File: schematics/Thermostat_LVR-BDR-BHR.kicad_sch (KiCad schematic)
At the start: 12 parts, among them J1 Dupont 6pin, J2 Dupont 6pin, SW1 Button Down, SW2 Button Up, SW3 Button Enter

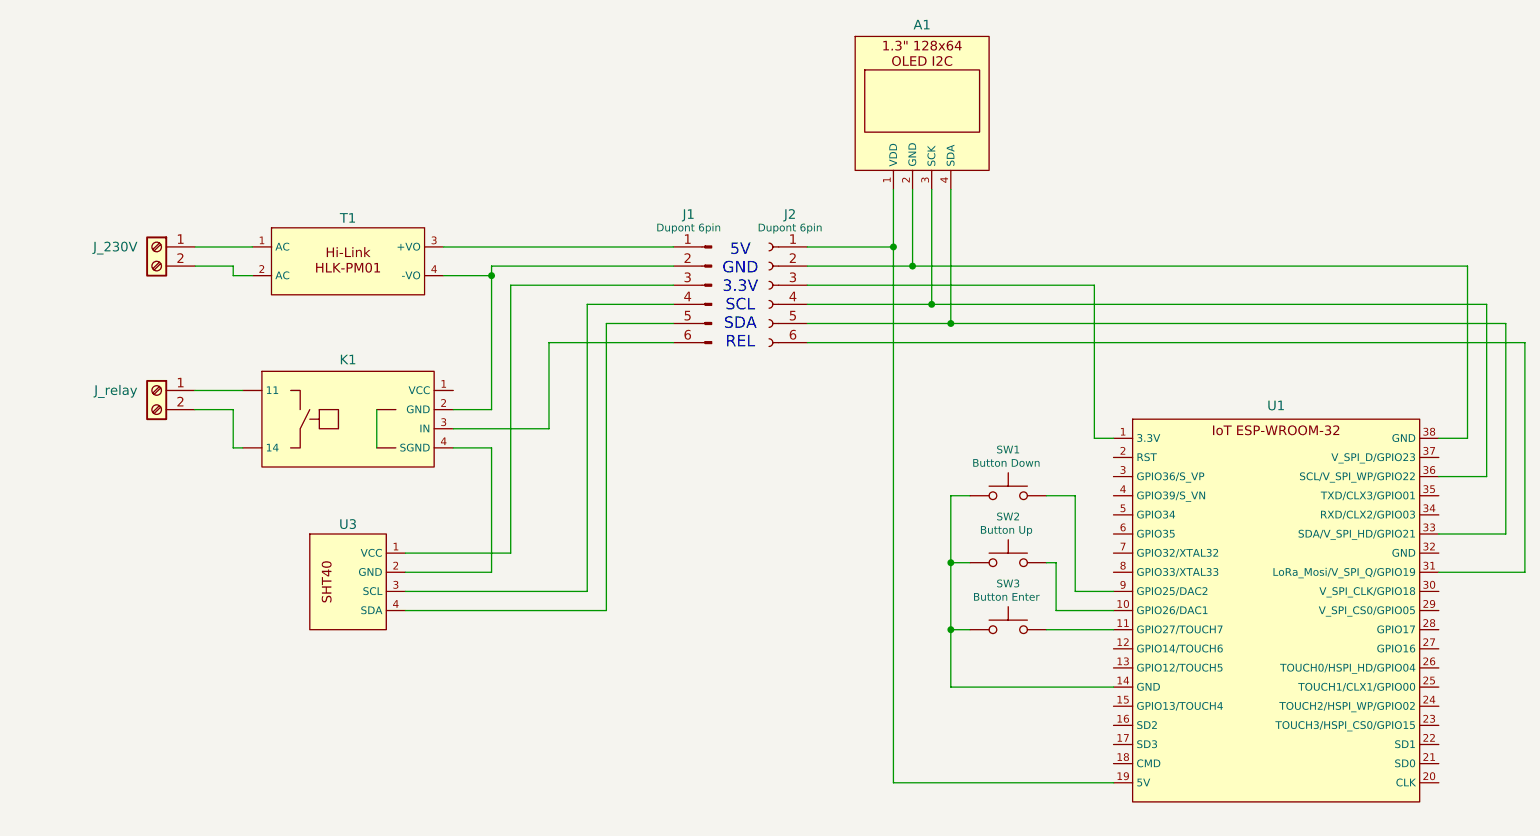
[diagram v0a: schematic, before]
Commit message: commit
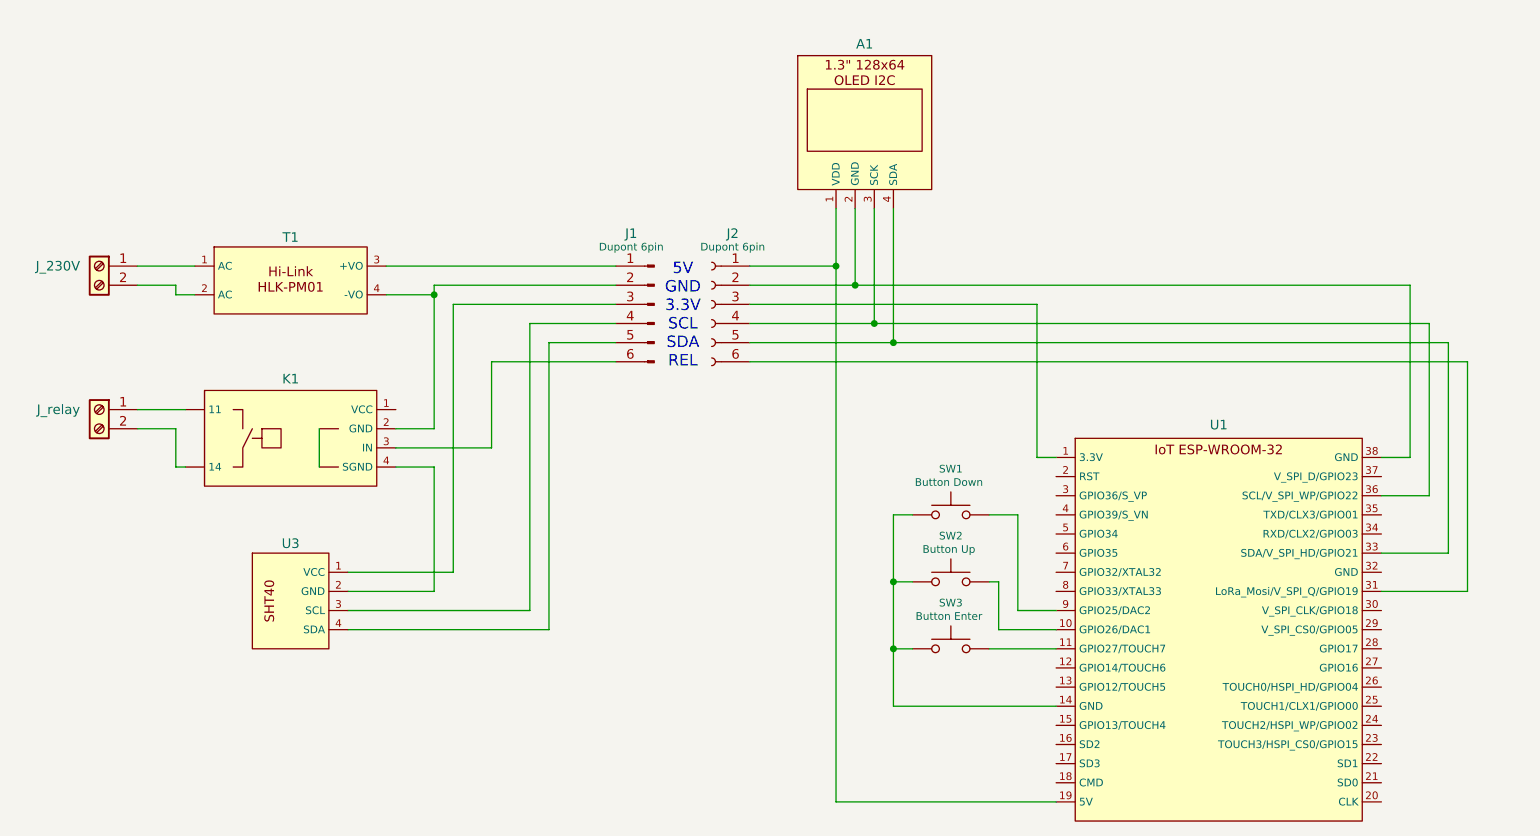
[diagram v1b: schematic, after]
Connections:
- net at K1.: now also J_relay.2 (Pin_2)
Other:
- title: (none) -> Themostat LVR, BDR, BHR
- moved on the sheet: A1, J1, J2, J_230V, J_relay, K1, SW1, SW2, SW3, T1, U1, U3
